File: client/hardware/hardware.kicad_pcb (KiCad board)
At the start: 2 copper layers, 60.8 x 42.5 mm, 58 parts, among them J1 Screw_Terminal_01x04, J2 EXT_COM, K1 G6H-2, M1 HC-12, Q1 2N7002, SW1 ADDRESS, SW2 CHANNEL, U1 XL1509-3.3, U2 TLV1117-33, U3 ESP32-C3_SUPERMINI_SMD

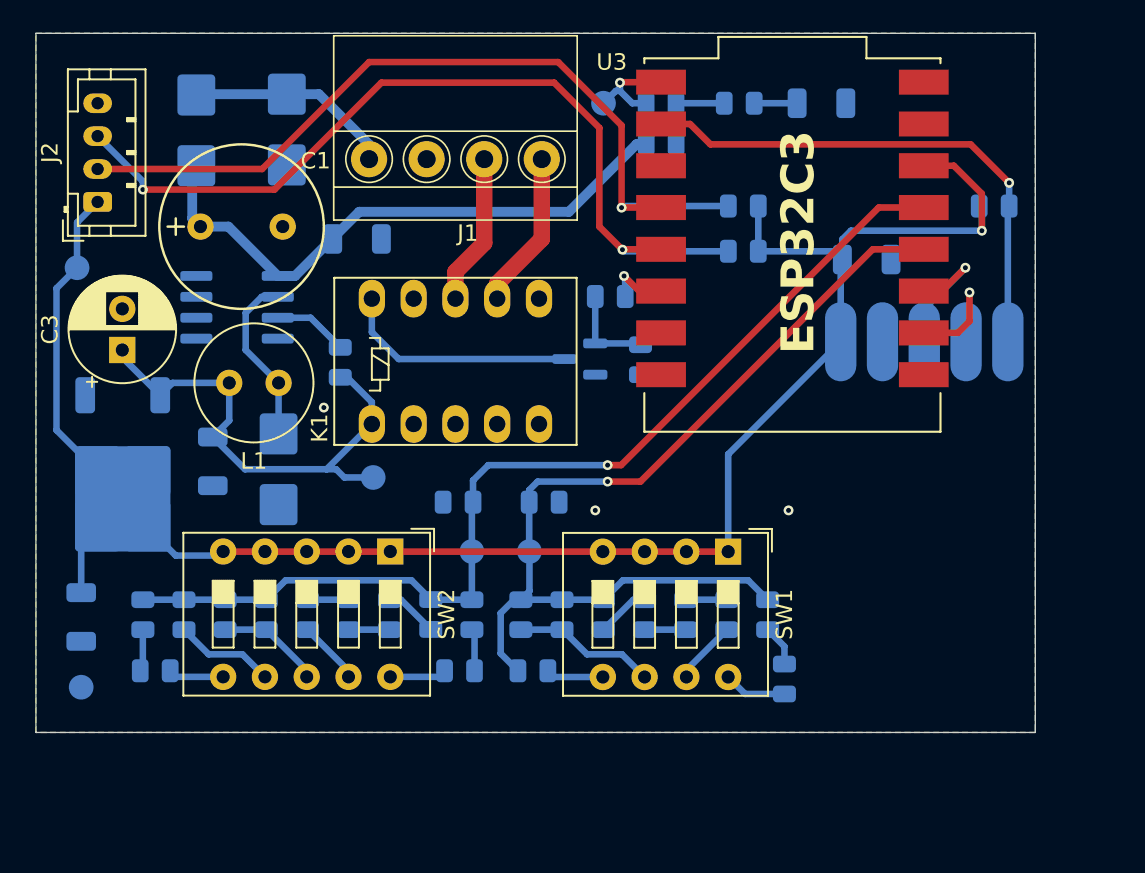
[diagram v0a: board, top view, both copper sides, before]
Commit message: hw
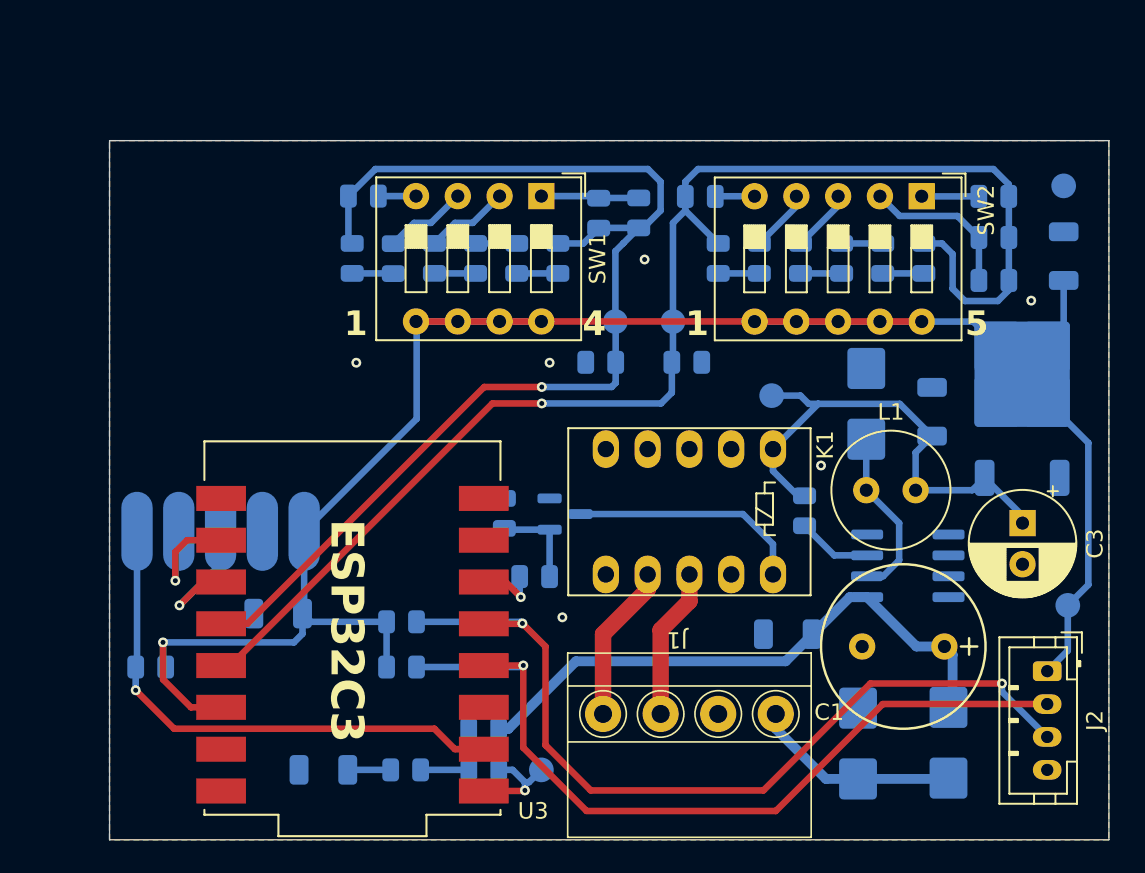
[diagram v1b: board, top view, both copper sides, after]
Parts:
- removed the R12 at (122.2, 88.8)
- removed the R23 at (99.2, 88.8)
- removed the R24 at (98.5, 85.3)
- added R14: 1kΩ, JLCPCB-Kicad-Footprints:R_0805, B.Cu at (132.4, 59.9)
- added R4: 1kΩ, JLCPCB-Kicad-Footprints:R_0805, B.Cu at (111.9, 59.9)
- moved TP3 67.1 mm to (154.5, 59.3), turned to 0 degrees
- moved J2 64.4 mm to (153.5, 88.8), turned to -90 degrees
- moved TP2 63.6 mm to (154.7, 84.8), turned to 0 degrees
- moved C5 63.6 mm to (154.5, 63.5), turned to 90 degrees
- moved D1 59.0 mm to (147.5, 93.1), turned to -90 degrees
- moved R25 58.4 mm to (99.0, 88.5), turned to 0 degrees
- moved C3 55.7 mm to (152.0, 79.8), turned to -90 degrees
- moved R23 55.4 mm to (150.2, 59.9), turned to 0 degrees
- moved U2 54.9 mm to (151.9, 72.0), turned to 90 degrees
- moved R21 52.1 mm to (150.2, 62.4), turned to 0 degrees
- moved D2 51.0 mm to (142.0, 93.2), turned to -90 degrees
- moved C7 50.6 mm to (109.5, 94.8), turned to 0 degrees
- moved R22 48.7 mm to (150.2, 65.0), turned to 0 degrees
- moved C1 47.6 mm to (144.7, 87.3), turned to 180 degrees
- moved R28 45.3 mm to (114.5, 94.8), turned to 0 degrees
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- renumbered R9 to R10, R10 to R11, R11 to R12, R14 to R15, R15 to R16, R16 to R17, R17 to R18, R18 to R19, R19 to R20, R20 to R21, R21 to R22, R22 to R23, R25 to R24, R26 to R25, R27 to R26, R29 to R27, R30 to R29, R31 to R30, R4 to R5, R5 to R6, R6 to R7, R7 to R8, R8 to R9
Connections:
- R11 pad 1: Net-(R10-Pad1) (its old number) -> Net-(R11-Pad1)
- R12 pad 1: Net-(R10-Pad1) (its old number) -> Net-(R11-Pad1)
- R15 pad 1: Net-(R14-Pad1) -> Net-(R15-Pad1)
- R17 pad 1: Net-(R16-Pad1) -> Net-(R17-Pad1)
- R21 pad 1: Net-(R20-Pad1) -> Net-(R21-Pad1)
- R22 pad 1: Net-(R20-Pad1) -> Net-(R21-Pad1)
- R23 pad 1: Net-(R22-Pad1) -> Net-(R23-Pad1)
- R5 pad 1: Net-(R4-Pad1) -> Net-(R5-Pad1)
- R7 pad 1: Net-(R6-Pad1) -> Net-(R7-Pad1)
- SW1 pad 1: +3.3V -> Net-(R11-Pad1)
- SW1 pad 2: +3.3V -> Net-(R7-Pad1)
- SW1 pad 3: +3.3V -> Net-(R5-Pad1)
- SW1 pad 4: +3.3V -> Net-(R4-Pad1)
- SW1 pad 5: Net-(R12-Pad1) -> +3.3V
- SW1 pad 6: Net-(R10-Pad1) (its old number) -> +3.3V
- SW1 pad 7: Net-(R6-Pad1) -> +3.3V
- SW1 pad 8: Net-(R4-Pad1) -> +3.3V
- SW2 pad 1: +3.3V -> Net-(R23-Pad1)
- SW2 pad 10: Net-(R14-Pad1) -> +3.3V
- SW2 pad 2: +3.3V -> Net-(R21-Pad1)
- SW2 pad 3: +3.3V -> Net-(R17-Pad1)
- SW2 pad 4: +3.3V -> Net-(R15-Pad1)
- SW2 pad 5: +3.3V -> Net-(R14-Pad1)
- SW2 pad 6: Net-(R23-Pad1) -> +3.3V
- SW2 pad 7: Net-(R22-Pad1) -> +3.3V
- SW2 pad 8: Net-(R20-Pad1) -> +3.3V
- SW2 pad 9: Net-(R16-Pad1) -> +3.3V
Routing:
- net CHANNEL_SET: track 62.5 -> 85.2 mm
- net +3.3V: track 109.0 -> 126.6 mm
- net ADDR_SET: track 58.4 -> 71.6 mm
- net Net-(R21-Pad1): track 0.00 -> 9.67 mm
- net Net-(R10-Pad1) (its old number): track 8.71 -> 0.00 mm
- net Net-(R20-Pad1): track 6.39 -> 0.00 mm
- net Net-(R11-Pad1): track 0.00 -> 6.12 mm
- net Net-(R22-Pad1): track 6.11 -> 0.00 mm
- net Net-(R5-Pad1): track 0.00 -> 5.53 mm
- net Net-(R7-Pad1): track 0.00 -> 5.15 mm
- net Net-(R16-Pad1): track 3.91 -> 0.00 mm
- net Net-(R6-Pad1): track 3.90 -> 0.00 mm
- net Net-(R17-Pad1): track 0.00 -> 3.82 mm
- net Net-(R15-Pad1): track 0.00 -> 3.80 mm
- net Net-(R12-Pad1): track 3.50 -> 0.00 mm
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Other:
- board size 60.8 x 42.5 mm -> 60.7 x 42.5 mm
- board text added: "1"
- board text added: "4"
- board text added: "5"
